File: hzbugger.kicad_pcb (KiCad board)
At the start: 2 copper layers, 55.4 x 26.7 mm, 54 parts, among them J2 IDC, J4 SWD, J6 GPIO, SW1 RESET_SW, SW2 BOOT0_SW, U1 STM32F103C8T6, U2 SRV05-4, U3 AMS1117-3.3, U4 HX AM 90D, Y1 8M

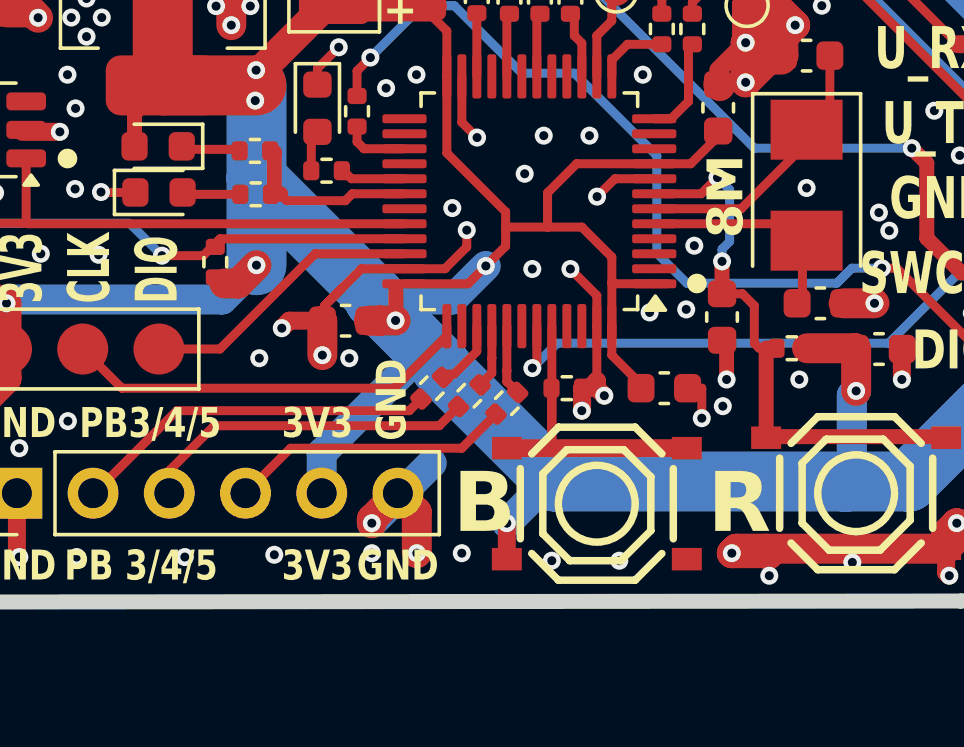
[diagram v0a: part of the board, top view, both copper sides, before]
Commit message: routing
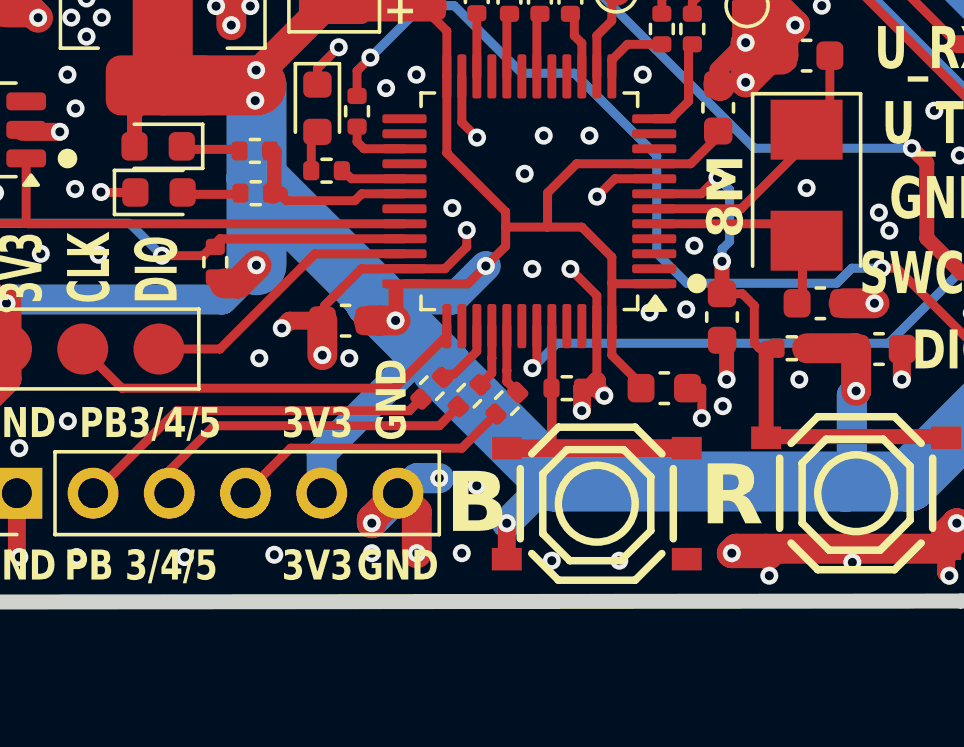
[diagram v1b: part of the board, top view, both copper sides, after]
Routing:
- net GND: vias 143 -> 145
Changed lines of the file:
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@@
 	(footprint "Resistor_SMD:R_0402_1005Metric"
 		(layer "F.Cu")
-		(at 124.1298 86.5378 180)
+		(at 124.1298 86.5 180)
 		(descr "Resistor SMD 0402 (1005 Metric), square (rectangular) end terminal, IPC_7351 nominal, (Body size source: IPC-SM-782 page 72, https://www.pcb-3d.com/wordpress/wp-content/uploads/ipc-sm-782a_amendment_1_and_2.pdf), generated with kicad-footprint-generator")
 		(tags "resistor")
@@
 	)
 	(gr_text "R"
-		(at 140.25 98 0)
+		(at 140 97.75 0)
 		(layer "F.SilkS")
 		(effects
@@
 	)
 	(gr_text "B"
-		(at 131.75 98 0)
+		(at 131.5 98 0)
 		(layer "F.SilkS")
 		(effects
@@
 	)
 	(via
+		(at 130.25 96)
+		(size 0.6)
+		(drill 0.3)
+		(layers "F.Cu" "B.Cu")
+		(net 9)
+	)
+	(via
 		(at 131.1656 87.7316)
 		(size 0.6)
@@
 	)
 	(via
+		(at 131.5 96.25)
+		(size 0.6)
+		(drill 0.3)
+		(layers "F.Cu" "B.Cu")
+		(free yes)
+		(net 9)
+	)
+	(via
 		(at 127.508 78.105)
 		(size 0.6)
@@
 	(segment
 		(start 128 97.5)
-		(end 130 95.5)
+		(end 129.5 96)
 		(width 1)
 		(layer "B.Cu")
@@
 	)
 	(segment
+		(start 129.5 96)
+		(end 130.25 96)
+		(width 1)
+		(layer "B.Cu")
+		(net 9)
+	)
+	(segment
 		(start 136 79.9)
 		(end 136.144 79.756)
@@
 	)
 	(segment
-		(start 124.6398 86.5378)
-		(end 124.9548 86.5378)
+		(start 127.434 86.75)
+		(end 127.665 86.519)
 		(width 0.3)
 		(layer "F.Cu")
@@
 	)
 	(segment
-		(start 127.349 86.519)
+		(start 127.665 86.519)
 		(end 129.089 86.519)
 		(width 0.3)
@@
 	)
 	(segment
-		(start 127.118 86.75)
-		(end 127.349 86.519)
-		(width 0.3)
-		(layer "F.Cu")
-		(net 45)
-	)
-	(segment
 		(start 125.167 86.75)
-		(end 127.118 86.75)
+		(end 127.434 86.75)
 		(width 0.3)
 		(layer "F.Cu")
@@
 	)
 	(segment
-		(start 121.756595 86.5378)
-		(end 121.693544 86.474749)
+		(start 124.6398 86.5)
+		(end 124.6776 86.5378)
+		(width 0.3)
+		(layer "F.Cu")
+		(net 45)
+	)
+	(segment
+		(start 124.6776 86.5378)
+		(end 124.9548 86.5378)
+		(width 0.3)
+		(layer "F.Cu")
+		(net 45)
+	)
+	(segment
+		(start 123.6198 86.5)
+		(end 123.582 86.5378)
 		(width 0.3)
 		(layer "F.Cu")
@@
 	)
 	(segment
-		(start 123.6198 86.5378)
+		(start 123.582 86.5378)
 		(end 121.756595 86.5378)
 		(width 0.3)
 		(layer "F.Cu")
+		(net 46)
+	)
+	(segment
+		(start 121.756595 86.5378)
+		(end 121.693544 86.474749)
+		(width 0.3)
+		(layer "F.Cu")
